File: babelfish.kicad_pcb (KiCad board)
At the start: 4 copper layers, 44.5 x 37.2 mm, 50 parts, among them J1 USB_C_Receptacle_USB2.0, J2 Conn_01x02, J3 SWD, J4 USB_C_Receptacle_USB2.0, J5 IO_A, J6 IO_B, U1 NCP1117-3.3_SOT223, U2 W25Q128JVS, U3 RP2040, U4 WS3232ECY, Y1 X322512MSB4SI

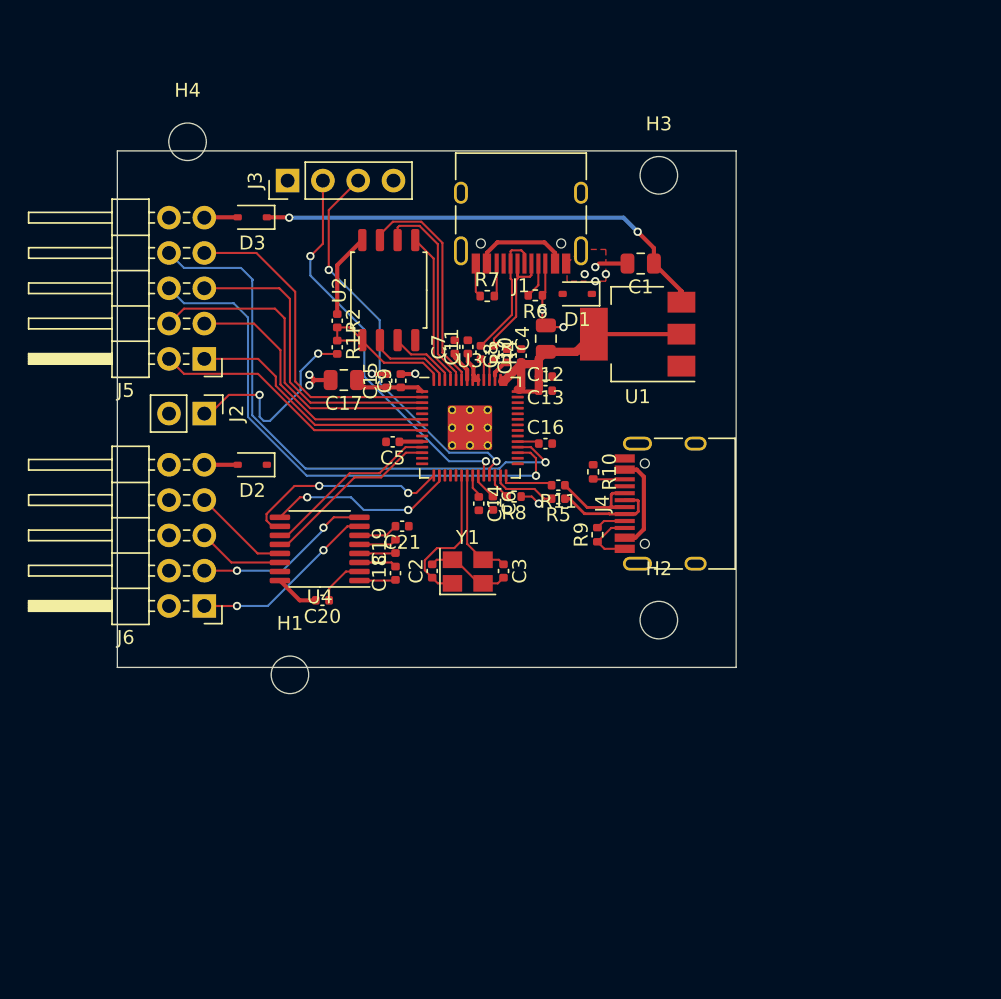
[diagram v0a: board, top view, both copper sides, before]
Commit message: updates
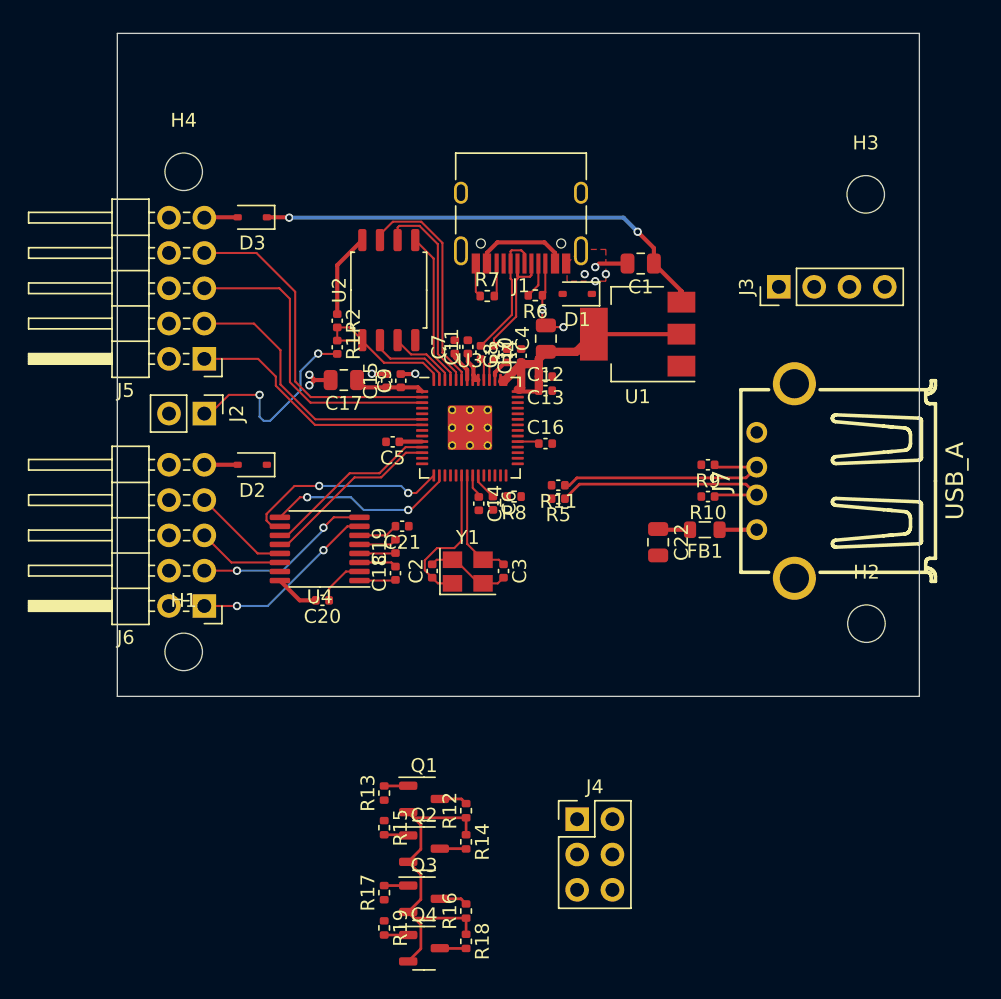
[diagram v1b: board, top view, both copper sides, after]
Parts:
- added C22: 10u, Capacitor_SMD:C_0805_2012Metric, F.Cu at (120.3, 106.2)
- added FB1: FerriteBead_Small, Inductor_SMD:L_0805_2012Metric, F.Cu at (123.7, 105.3)
- added J7: USB_A, RP2040_minimal:USB-A-TH__USB-AF-90, F.Cu at (128.8, 101.8)
- added Q1: ~, Package_TO_SOT_SMD:SOT-23-3, F.Cu at (103.5, 124.6)
- added Q2: ~, Package_TO_SOT_SMD:SOT-23-3, F.Cu at (103.5, 128.2)
- added Q3: ~, Package_TO_SOT_SMD:SOT-23-3, F.Cu at (103.5, 131.8)
- added Q4: ~, Package_TO_SOT_SMD:SOT-23-3, F.Cu at (103.5, 135.4)
- added R12: 10k, Resistor_SMD:R_0402_1005Metric, F.Cu at (106.5, 125.5)
- added R13: 10k, Resistor_SMD:R_0402_1005Metric, F.Cu at (100.6, 124.2)
- added R14: 10k, Resistor_SMD:R_0402_1005Metric, F.Cu at (106.5, 127.7)
- added R15: 10k, Resistor_SMD:R_0402_1005Metric, F.Cu at (100.6, 126.7)
- added R16: 10k, Resistor_SMD:R_0402_1005Metric, F.Cu at (106.5, 132.7)
- added R17: 10k, Resistor_SMD:R_0402_1005Metric, F.Cu at (100.6, 131.4)
- added R18: 10k, Resistor_SMD:R_0402_1005Metric, F.Cu at (106.5, 134.9)
- added R19: 10k, Resistor_SMD:R_0402_1005Metric, F.Cu at (100.6, 133.9)
- J1: value USB_C_Receptacle_USB2.0 -> TYPE-C-31-M-12
- J4: value USB_C_Receptacle_USB2.0 -> Shifter Power; footprint Connector_USB:USB_C_Receptacle_HRO_TYPE-C-31-M-12 -> Connector_PinHeader_2.54mm:PinHeader_2x03_P2.54mm_Vertical
- R10, R9: value 5.1K -> 15k; footprint Resistor_SMD:R_0402_1005Metric -> Capacitor_SMD:C_0402_1005Metric
- R11, R5: value 27 -> 22
- moved J3 36.2 mm to (129.0, 87.8)
- moved J4 23.9 mm to (114.5, 126.1), turned to 0 degrees
- moved H3 14.9 mm to (135.3, 81.1)
- moved H2 14.9 mm to (135.3, 112.0)
- moved R9 9.41 mm to (123.9, 100.6), turned to 180 degrees
- moved R10 8.45 mm to (123.9, 102.9), turned to 180 degrees
- moved H1 7.82 mm to (86.2, 114.0)
- moved H4 2.18 mm to (86.2, 79.5)
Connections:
- J5 pad 2: /GPIO6 -> /U1_RX_CH
- J5 pad 4: /GPIO2 -> /U1_TX_CH
- J5 pad 6: /GPIO20 -> /U0_RX_CH
- J5 pad 8: /GPIO21 -> /U0_TX_CH
- R10 pad 1: GND -> /USB2_D-
- R10 pad 2: Net-(J4-CC2) -> GND
- R11 pad 2: /GPIO17 -> /GPIO15
- R5 pad 2: /GPIO16 -> /GPIO14
- R8 pad 1: +3V3 -> /RUN
- R8 pad 2: /RUN -> +3V3
- R9 pad 1: GND -> /USB2_D+
- R9 pad 2: Net-(J4-CC1) -> GND
- U3 pad 27: /GPIO16 -> /U0_TX_C
- U3 pad 28: /GPIO17 -> /U0_RX_C
- U3 pad 31: /GPIO20 -> /U1_TX_C
- U3 pad 32: /GPIO21 -> /U1_RX_C
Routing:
- net /GPIO21: track 42.0 -> 0.00 mm, vias 1 -> 0
- net /GPIO20: track 38.9 -> 0.00 mm, vias 1 -> 0
- net /SWD: track 29.1 -> 0.00 mm, vias 2 -> 0
- net /SWCLK: track 28.4 -> 0.00 mm, vias 2 -> 0
- net /GPIO2: track 24.3 -> 0.00 mm
- net +3.3V: track 0.00 -> 24.1 mm
- net /GPIO6: track 20.3 -> 0.00 mm
- net /USB2_D-: track 7.57 -> 17.6 mm
- net /USB2_D+: track 7.84 -> 17.4 mm
- net /GPIO16: track 4.69 -> 0.00 mm
- net VBUS: track 14.1 -> 9.38 mm
- net GND: track 26.5 -> 21.9 mm
- net /GPIO17: track 3.88 -> 0.00 mm
- net Net-(J7-VBUS): track 0.00 -> 2.68 mm
- net Net-(J4-CC2): track 2.28 -> 0.00 mm
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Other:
- board size 44.5 x 37.2 mm -> 57.7 x 47.7 mm

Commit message: rev 0.1
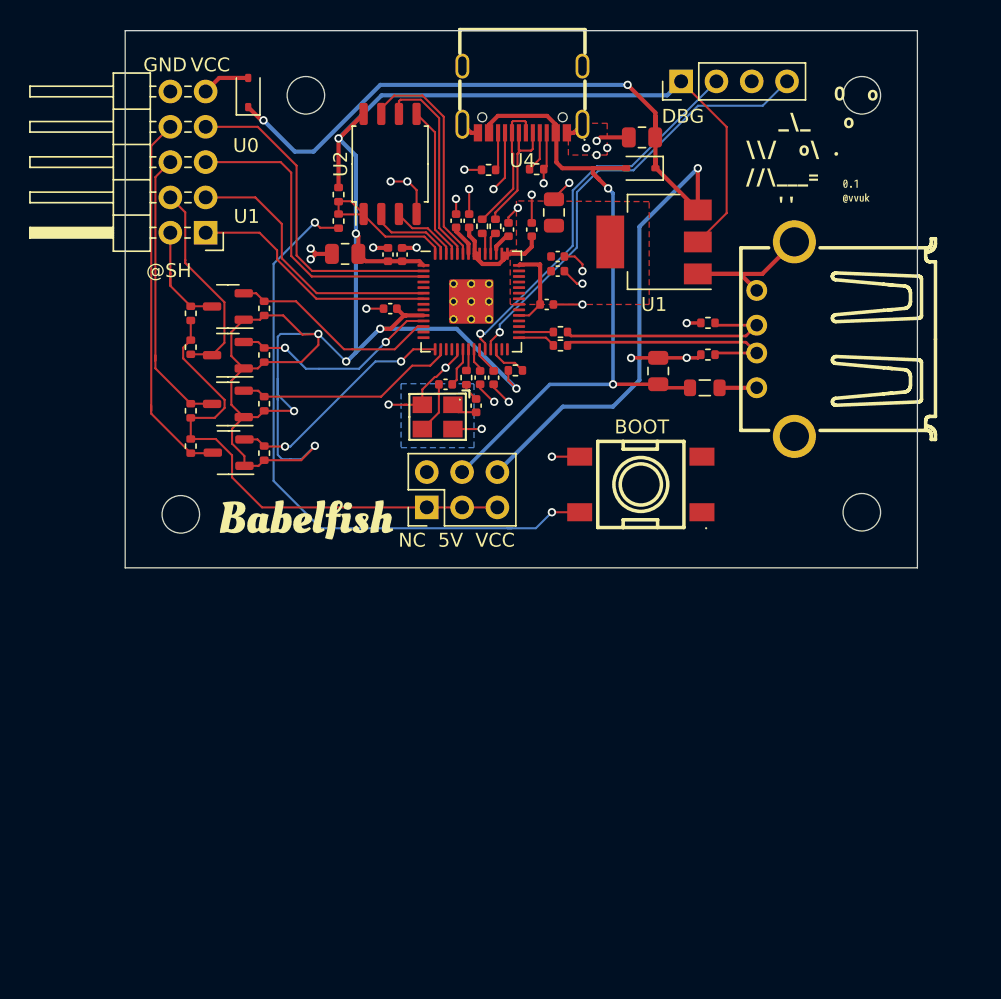
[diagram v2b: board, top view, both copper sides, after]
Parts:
- removed C18, C19, C20, C21: 0.1uf, Capacitor_SMD:C_0402_1005Metric
- removed D2: 1N5819WS, Diode_SMD:D_SOD-323
- removed J1: TYPE-C-31-M-12, Connector_USB:USB_C_Receptacle_HRO_TYPE-C-31-M-12
- removed J2: Conn_01x02, Connector_PinHeader_2.54mm:PinHeader_1x02_P2.54mm_Vertical
- removed J6: IO_B, Connector_PinHeader_2.54mm:PinHeader_2x05_P2.54mm_Horizontal
- removed Y1: X322512MSB4SI, Crystal:Crystal_SMD_3225-4Pin_3.2x2.5mm
- added R20: 1k, Resistor_SMD:R_0402_1005Metric, F.Cu at (106.5, 94.3)
- added SW1: K2-1156SP-D5SW-05, lcsc:SW-SMD_4P-L6.3-W6.2-P4.00-LS9.4-TL, F.Cu at (119.1, 102.0)
- added X1: X322512MSB4SI, lcsc:OSC-SMD_4P-L3.2-W2.5-BL, F.Cu at (104.5, 97.1)
- added kibuzzard-644F3679: G***, kibuzzard-644F3679, F.Cu at (95.0, 104.5)
- added kibuzzard-644F39EB: G***, kibuzzard-644F39EB, F.Cu at (131.4, 77.5)
- added kibuzzard-644F3A2B: G***, kibuzzard-644F3A2B, F.Cu at (134.6, 80.9)
- C2, C3: value 32p -> 30p
- Q1: value ~ -> BSS138
- R1, R10, R11, R2, R3, R4, R5, R9: footprint Capacitor_SMD:C_0402_1005Metric -> Resistor_SMD:R_0402_1005Metric
- U4: value WS3232ECY -> GT-USB-7010ASV; footprint Package_SO:TSSOP-16_4.4x5mm_P0.65mm -> lcsc:USB-C-SMD_G-SWITCH_GT-USB-7010ASV
- moved Q4 48.3 mm to (89.4, 89.2), turned to 180 degrees
- moved R18 47.8 mm to (92.0, 89.3), turned to 90 degrees
- moved R19 46.4 mm to (86.7, 89.7), turned to 90 degrees
- moved R16 42.6 mm to (92.0, 92.7)
- moved R17 41.6 mm to (86.7, 92.1), turned to -90 degrees
- moved Q3 41.6 mm to (89.4, 92.7), turned to 180 degrees
- moved U4 35.5 mm to (110.6, 74.3)
- moved Q2 35.0 mm to (89.4, 96.2), turned to 180 degrees
- moved R14 34.7 mm to (92.0, 96.2), turned to 90 degrees
- moved R15 33.1 mm to (86.7, 96.7), turned to 90 degrees
- moved R12 29.5 mm to (92.0, 99.7)
- moved Q1 28.6 mm to (89.4, 99.7), turned to 180 degrees
- moved R13 28.6 mm to (86.7, 99.2), turned to -90 degrees
- moved J4 24.9 mm to (103.7, 103.7), turned to 90 degrees
- moved J3 16.4 mm to (122.0, 73.0)
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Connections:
- net Net-(D3-A) renamed /VCC_IN
- C2 pad 1: /XIN -> Net-(X1-OSC1)
- C2 pad 2: GND -> Net-(C2-Pad2)
- C3 pad 1: /XOUT -> Net-(X1-OSC2)
- C3 pad 2: GND -> /XIN
- J3 pad 3: /SWD -> GND
- J3 pad 4: GND -> /SWD
- J4 pad 1: Net-(J4-Pin_1) -> /SH_REF
- J4 pad 3: Net-(J4-Pin_1) -> /SH_REF
- J4 pad 5: Net-(J4-Pin_1) -> /SH_REF
- J4 pad 6: +3V3 -> VCC
- Q1 pad 1: /U0_TX_CH -> +3V3
- Q1 pad 2: +3.3V -> /U0_TX_B
- Q1 pad 3: /U0_TX_C -> /U0_TX_CH
- Q2 pad 1: /U0_RX_CH -> +3V3
- Q2 pad 2: +3.3V -> /U0_RX_B
- Q2 pad 3: /U0_RX_C -> /U0_RX_CH
- Q3 pad 1: /U1_TX_CH -> +3V3
- Q3 pad 2: +3.3V -> /U1_TX_B
- Q3 pad 3: /U1_TX_C -> /U1_TX_CH
- Q4 pad 1: /U1_RX_CH -> +3V3
- Q4 pad 2: +3.3V -> /U1_RX_B
- Q4 pad 3: /U1_RX_C -> /U1_RX_CH
- R11 pad 2: /GPIO15 -> /GPIO19
- R12 pad 1: +3.3V -> +3V3
- R12 pad 2: /U0_TX_C -> /U0_TX_B
- R13 pad 1: unconnected-(R13-Pad1) -> /SH_REF
- R14 pad 1: +3.3V -> +3V3
- R14 pad 2: /U0_RX_C -> /U0_RX_B
- R15 pad 1: unconnected-(R15-Pad1) -> /SH_REF
- R16 pad 1: +3.3V -> +3V3
- R16 pad 2: /U1_TX_C -> /U1_TX_B
- R17 pad 1: unconnected-(R17-Pad1) -> /SH_REF
- R18 pad 1: +3.3V -> +3V3
- R18 pad 2: /U1_RX_C -> /U1_RX_B
- R19 pad 1: unconnected-(R19-Pad1) -> /SH_REF
- R5 pad 2: /GPIO14 -> /GPIO18
- R6 pad 1: GND -> Net-(U4-CC1)
- R6 pad 2: Net-(J1-CC1) -> GND
- R7 pad 1: GND -> Net-(U4-CC2)
- R7 pad 2: Net-(J1-CC2) -> GND
- U4 pad 1: Net-(U4-C1+) -> GND
- U4 pad 2: Net-(U4-V+) -> GND
- U4 pad 3: Net-(U4-C1-) -> GND
- U4 pad 4: Net-(U4-C2+) -> GND
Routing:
- net +3V3: track 42.2 -> 163.5 mm, vias 0 -> 8
- net GND: track 21.9 -> 72.5 mm, vias 10 -> 31
- net VCC: track 33.8 -> 76.9 mm, vias 2 -> 3
- net VBUS: track 9.38 -> 51.0 mm, vias 0 -> 2
- net /SH_REF: track 0.00 -> 37.0 mm
- net /SWD: track 0.00 -> 32.3 mm, vias 0 -> 1
- net /~{USB_BOOT}: track 14.6 -> 46.1 mm
- net /SWCLK: track 0.00 -> 28.1 mm, vias 0 -> 1
- net /U0_TX_CH: track 1.73 -> 27.2 mm
- net +3.3V: track 24.1 -> 0.00 mm
- net /U0_RX_CH: track 1.75 -> 20.8 mm
- net /U0_232_TX: track 13.5 -> 0.00 mm, vias 2 -> 0
- net /U1_TX_CH: track 1.73 -> 14.9 mm
- net /U0_232_RX: track 12.8 -> 0.00 mm, vias 2 -> 0
- net /XIN: track 11.0 -> 2.84 mm
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- added copper zone on B.Cu, net (none)
- added copper zone on F.Cu, net +3V3
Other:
- board size 57.7 x 47.7 mm -> 57 x 38.7 mm
- rule pad_to_mask_clearance: 0.051 -> 0
- board text added: "@SH"
- board text added: "BOOT"
- board text added: "DBG"
- board text added: "GND"
- board text added: "NC 5V VCC"
- board text added: "U0"
- board text added: "U1"
- board text added: "VCC"

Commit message: rev2, pre review
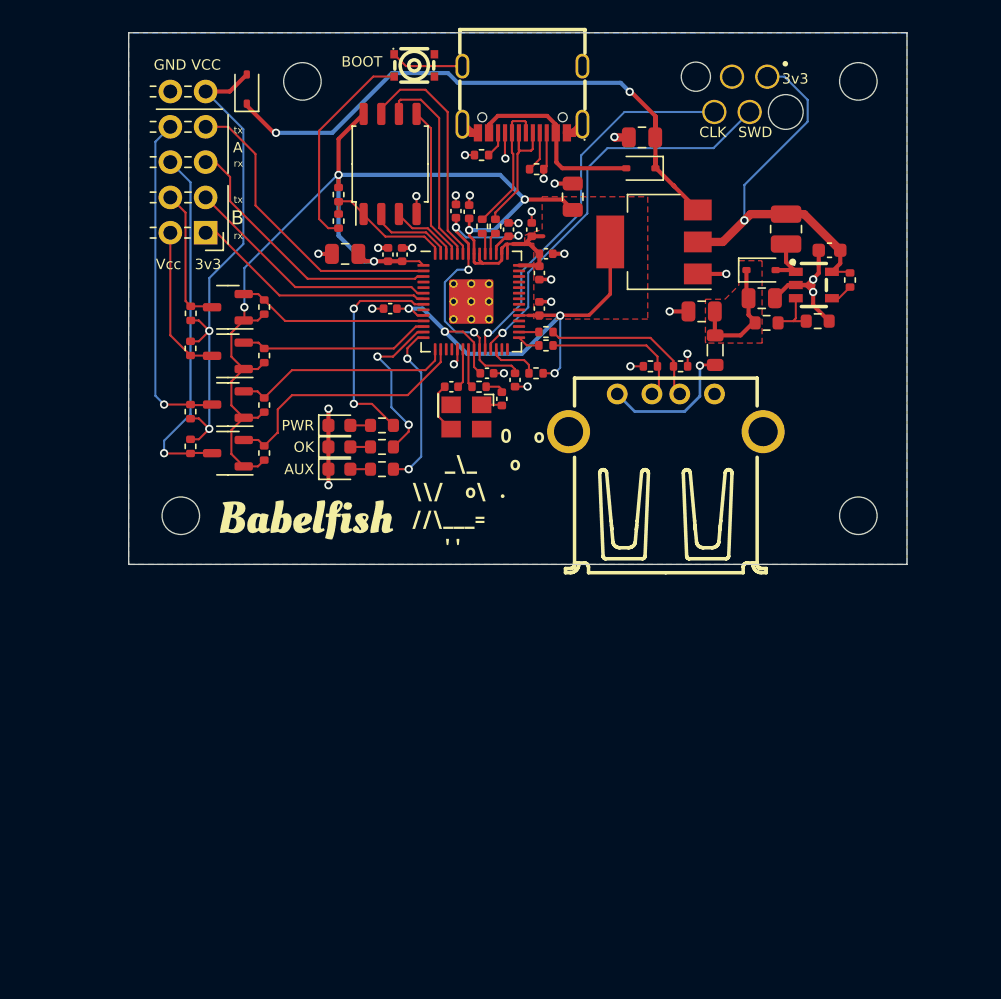
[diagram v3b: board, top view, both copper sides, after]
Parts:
- removed J4: Shifter Power, Connector_PinHeader_2.54mm:PinHeader_2x03_P2.54mm_Vertical
- removed kibuzzard-644F3A2B: G***, kibuzzard-644F3A2B
- added C18: 4u7, Capacitor_SMD:C_0603_1608Metric, F.Cu at (132.7, 85.2)
- added C19: 10u, Capacitor_SMD:C_0805_2012Metric, F.Cu at (127.8, 88.6)
- added D2: Red, LED_SMD:LED_0603_1608Metric, F.Cu at (97.4, 97.8)
- added D4: Red, LED_SMD:LED_0603_1608Metric, F.Cu at (97.4, 99.3)
- added D5: Blue, LED_SMD:LED_0603_1608Metric, F.Cu at (97.4, 100.9)
- added D6: 40V/5A, Diode_SMD:D_SOD-323, F.Cu at (127.8, 86.6)
- added L1: 4u7, Inductor_SMD:L_1008_2520Metric, F.Cu at (129.6, 83.6)
- added R21: 68, Resistor_SMD:R_0603_1608Metric, F.Cu at (100.5, 97.8)
- added R22: 68, Resistor_SMD:R_0603_1608Metric, F.Cu at (100.5, 99.3)
- added R23: 68, Resistor_SMD:R_0603_1608Metric, F.Cu at (100.5, 100.9)
- added R24: 47k, Resistor_SMD:R_0603_1608Metric, F.Cu at (128.2, 90.4)
- added R25: 15k, Resistor_SMD:R_0603_1608Metric, F.Cu at (131.8, 90.2)
- added R26: 10k, Resistor_SMD:R_0402_1005Metric, F.Cu at (134.2, 87.3)
- added U5: LGS6302, lcsc:SOT-23-5_L3.0-W1.6-P0.95-LS2.8-BL, F.Cu at (131.6, 87.7)
- J3: footprint Connector_PinHeader_2.54mm:PinHeader_1x04_P2.54mm_Vertical -> SnapEDA:490107670412
- SW1: value K2-1156SP-D5SW-05 -> K2-1836UQ-C3DW-06; footprint lcsc:SW-SMD_4P-L6.3-W6.2-P4.00-LS9.4-TL -> lcsc:SW-SMD_4P-L2.8-W2.4-P1.60-LS3.0
- U3: renamed from U1; value NCP1117-3.3_SOT223 -> AMS1117-3.3
- moved kibuzzard-644F39EB 34.4 mm to (107.4, 102.2)
- moved SW1 34.3 mm to (102.8, 71.8), turned to 0 degrees
- moved J7 9.51 mm to (120.9, 96.8), turned to 0 degrees
- moved C22 5.31 mm to (123.5, 89.5), turned to 180 degrees
- moved J3 4.39 mm to (126.3, 73.9), turned to 0 degrees
- moved R10 4.22 mm to (119.8, 93.5)
- moved R9 3.70 mm to (122.0, 93.5), turned to 0 degrees
- moved Q4 3.55 mm to (89.4, 92.7)
- moved R14 3.54 mm to (92.0, 99.7)
- moved Q2 3.54 mm to (89.4, 99.8)
- moved Q1 3.46 mm to (89.4, 96.2)
- moved R12 3.46 mm to (92.0, 96.3)
- moved R16 3.45 mm to (92.0, 89.2)
- moved Q3 3.45 mm to (89.4, 89.2)
- moved R18 3.40 mm to (92.0, 92.7)
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- renumbered U3 to U1
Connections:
- net Net-(C2-Pad2) renamed /OSC1R
- net Net-(X1-OSC1) renamed /OSC1
- net Net-(X1-OSC2) renamed /OSC2
- C22 pad 1: VBUS -> +5V
- FB1 pad 2: VBUS -> +5V
- J3 pad 2: /SWCLK -> /SWD
- J3 pad 4: /SWD -> /SWCLK
- R13 pad 1: /SH_REF -> /VCC_IN
- R15 pad 1: /SH_REF -> /VCC_IN
- R17 pad 1: /SH_REF -> /VCC_IN
- R19 pad 1: /SH_REF -> /VCC_IN
- U1 pad 13: /GPIO10 -> /LED_P_OK
- U1 pad 14: /GPIO11 -> /LED_AUX
- U1 pad 8: /GPIO6 -> /LED_PWR
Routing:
- net /SH_REF: track 37.0 -> 0.00 mm
- net VBUS: track 51.0 -> 14.3 mm, vias 2 -> 0
- net VCC: track 76.9 -> 43.7 mm, vias 3 -> 2
- net /VCC_IN: track 3.47 -> 36.5 mm, vias 0 -> 2
- net /~{USB_BOOT}: track 46.1 -> 15.0 mm, vias 2 -> 0
- net +1V1: track 5.62 -> 23.5 mm, vias 0 -> 4
- net /LED_PWR: track 0.00 -> 15.7 mm, vias 0 -> 2
- net /LED_AUX: track 0.00 -> 12.1 mm, vias 0 -> 2
- net /LED_P_OK: track 0.00 -> 11.9 mm, vias 0 -> 2
- net +5V: track 0.00 -> 9.13 mm
- net +3V3: track 163.5 -> 155.2 mm, vias 8 -> 10
- net Net-(J7-VBUS): track 2.68 -> 10.2 mm, vias 0 -> 1
- net GND: track 72.5 -> 65.2 mm, vias 31 -> 28
- net /USB2_D-: track 17.1 -> 10.8 mm
- net /USB2_D+: track 17.2 -> 12.1 mm
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- added copper zone on F.Cu, net +5V
- added copper zone on B.Cu, net GND
- removed copper zone on B.Cu, net (none)
- removed copper zone on In2.Cu, net +3V3
- removed copper zone on F.Cu, net GND
- removed copper zone on In1.Cu, net GND
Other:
- board size 57 x 38.7 mm -> 56 x 38.2 mm
- copper layers 4 -> 2
- board text added: "3v3"
- board text added: "A"
- board text added: "AUX"
- board text added: "B"
- board text added: "CLK"
- board text added: "OK"
- board text added: "PWR"
- board text added: "SWD"
- board text added: "Vcc"
- board text added: "rx"
- board text added: "tx"
- board text removed: "@SH"
- board text removed: "DBG"
- board text removed: "NC 5V VCC"
- board text removed: "Stackup: JLC3313"
- board text removed: "U0"
- board text removed: "U1"
